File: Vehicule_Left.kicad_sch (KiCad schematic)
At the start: 16 parts, among them Q19 IRLZ44N, U4 LM339

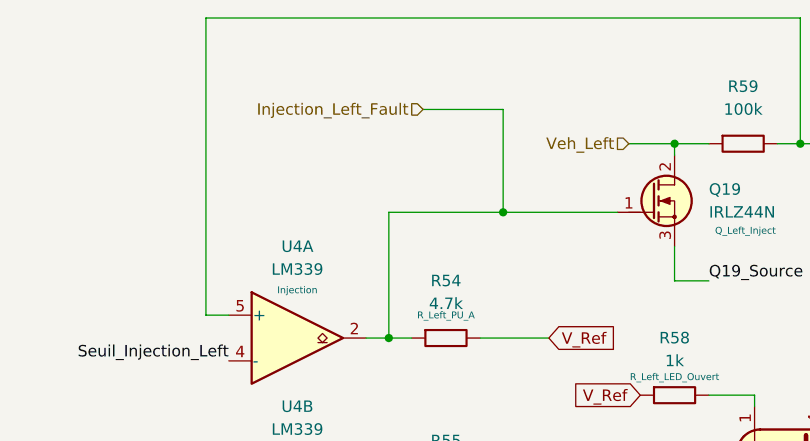
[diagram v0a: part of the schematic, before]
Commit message: Add files via upload
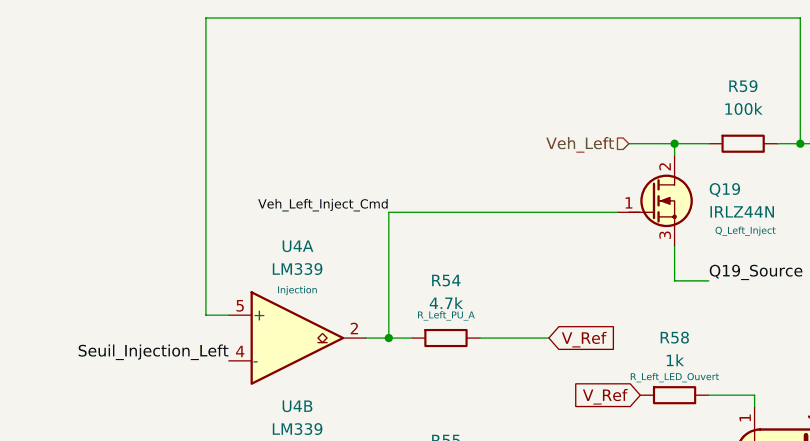
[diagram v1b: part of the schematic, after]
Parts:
- R61, R62, R63: footprint TRIM_3296W1103LF:TRIM_3296W1103LF -> (none)
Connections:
- net Injection_Left_Fault renamed Veh_Left_Inject_Cmd
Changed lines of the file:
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@@
-	)
-	(junction
-		(at 99.06 39.37)
-		(diameter 0)
-		(color 0 0 0 0)
 	)
 	(junction
@@
 	(wire
 		(pts
-			(xy 90.17 27.94) (xy 99.06 27.94)
-		)
-		(stroke
-			(width 0)
-			(type default)
-		)
-	)
-	(wire
-		(pts
 			(xy 106.68 71.12) (xy 127 71.12)
 		)
@@
 	(wire
 		(pts
-			(xy 86.36 39.37) (xy 99.06 39.37)
-		)
-		(stroke
-			(width 0)
-			(type default)
-		)
-	)
-	(wire
-		(pts
-			(xy 99.06 27.94) (xy 99.06 39.37)
+			(xy 86.36 39.37) (xy 111.76 39.37)
 		)
 		(stroke
@@
 		(pts
 			(xy 102.87 87.63) (xy 102.87 92.71)
-		)
-		(stroke
-			(width 0)
-			(type default)
-		)
-	)
-	(wire
-		(pts
-			(xy 99.06 39.37) (xy 111.76 39.37)
 		)
 		(stroke
@@
 			)
 			(justify left bottom)
+		)
+	)
+	(label "Veh_Left_Inject_Cmd"
+		(at 86.36 39.37 180)
+		(effects
+			(font
+				(size 1.016 1.016)
+			)
+			(justify right bottom)
 		)
 	)
@@
 		(shape input)
 		(at 113.03 31.75 180)
-		(effects
-			(font
-				(size 1.27 1.27)
-			)
-			(justify right)
-		)
-	)
-	(hierarchical_label "Injection_Left_Fault"
-		(shape input)
-		(at 90.17 27.94 180)
 		(effects
 			(font
@@
 			)
 		)
-		(property "Footprint" "TRIM_3296W1103LF:TRIM_3296W1103LF"
+		(property "Footprint" ""
 			(at 172.72 67.31 0)
 			(hide yes)
@@
 			)
 		)
-		(property "Footprint" "TRIM_3296W1103LF:TRIM_3296W1103LF"
+		(property "Footprint" ""
 			(at 172.72 48.26 0)
 			(hide yes)
@@
 			)
 		)
-		(property "Footprint" "TRIM_3296W1103LF:TRIM_3296W1103LF"
+		(property "Footprint" ""
 			(at 172.72 30.48 0)
 			(hide yes)
